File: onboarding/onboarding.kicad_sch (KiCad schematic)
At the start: 15 parts, among them IC1 ISL29125IROZ-T7, J1 Conn_01x05_Pin

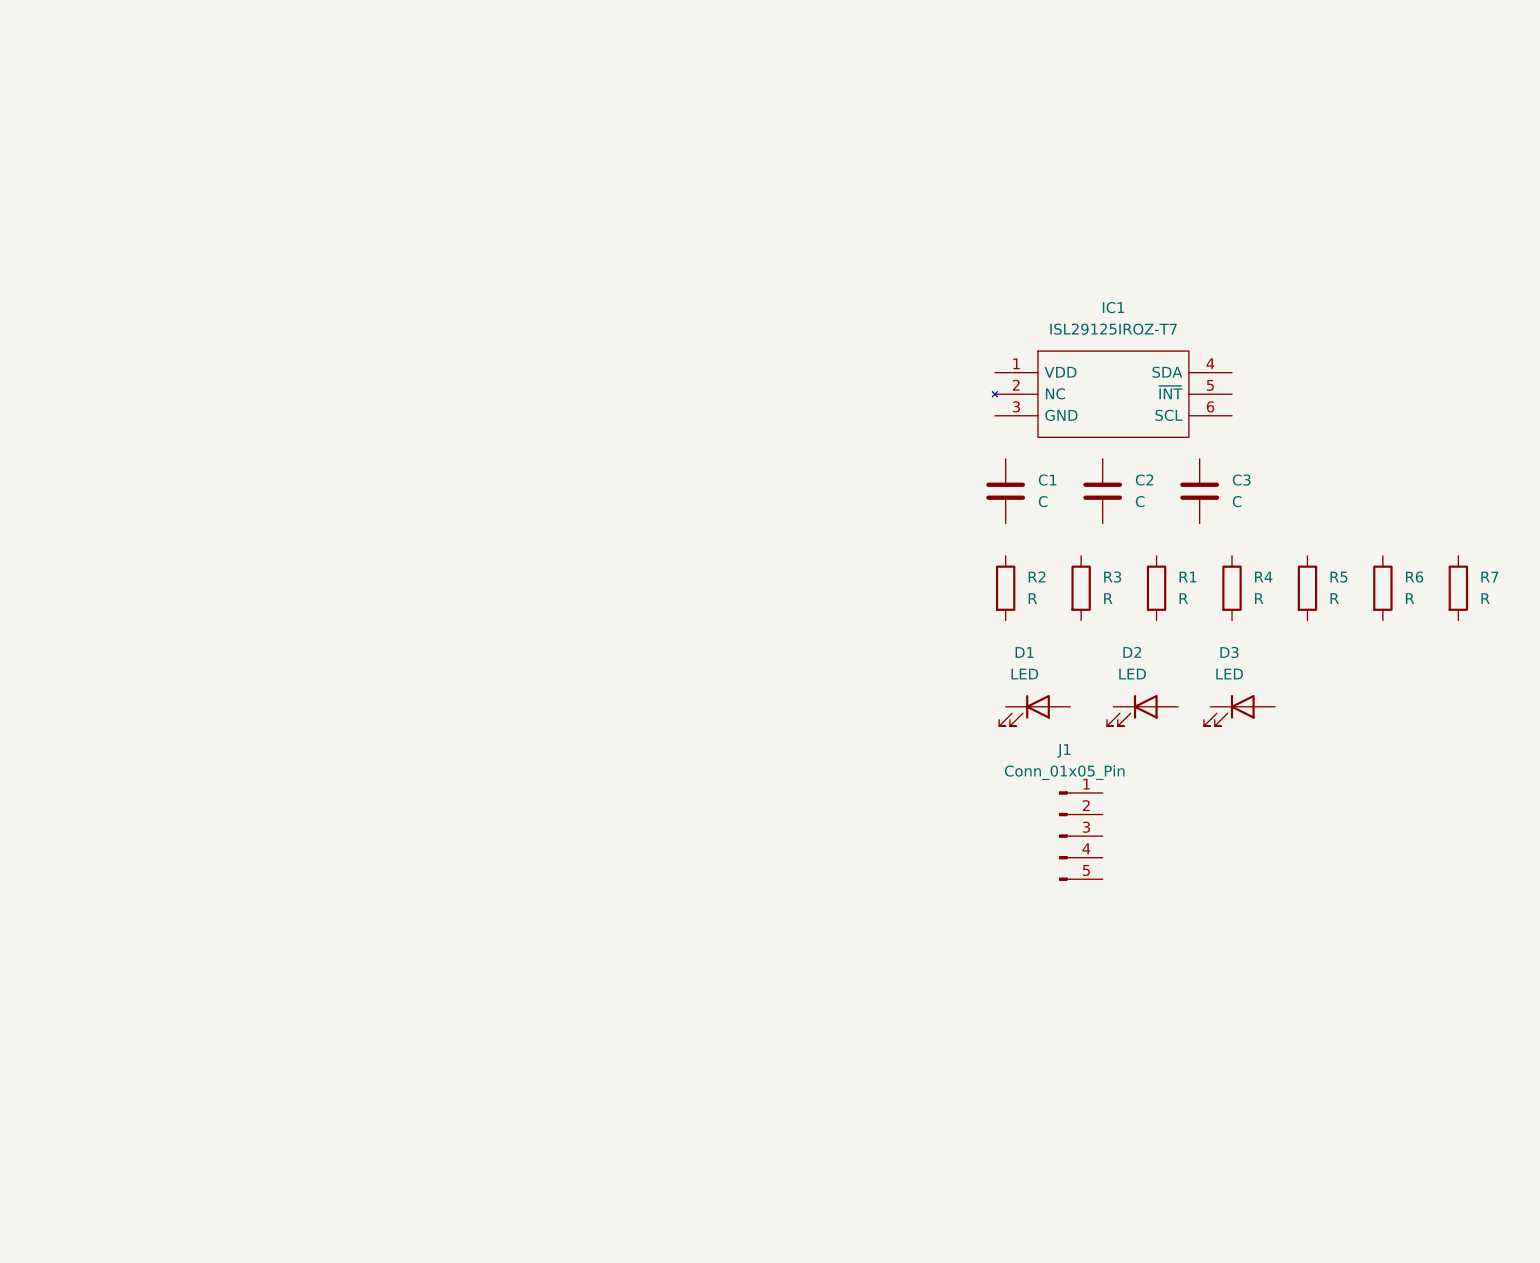
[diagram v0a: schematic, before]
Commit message: finished onboarding
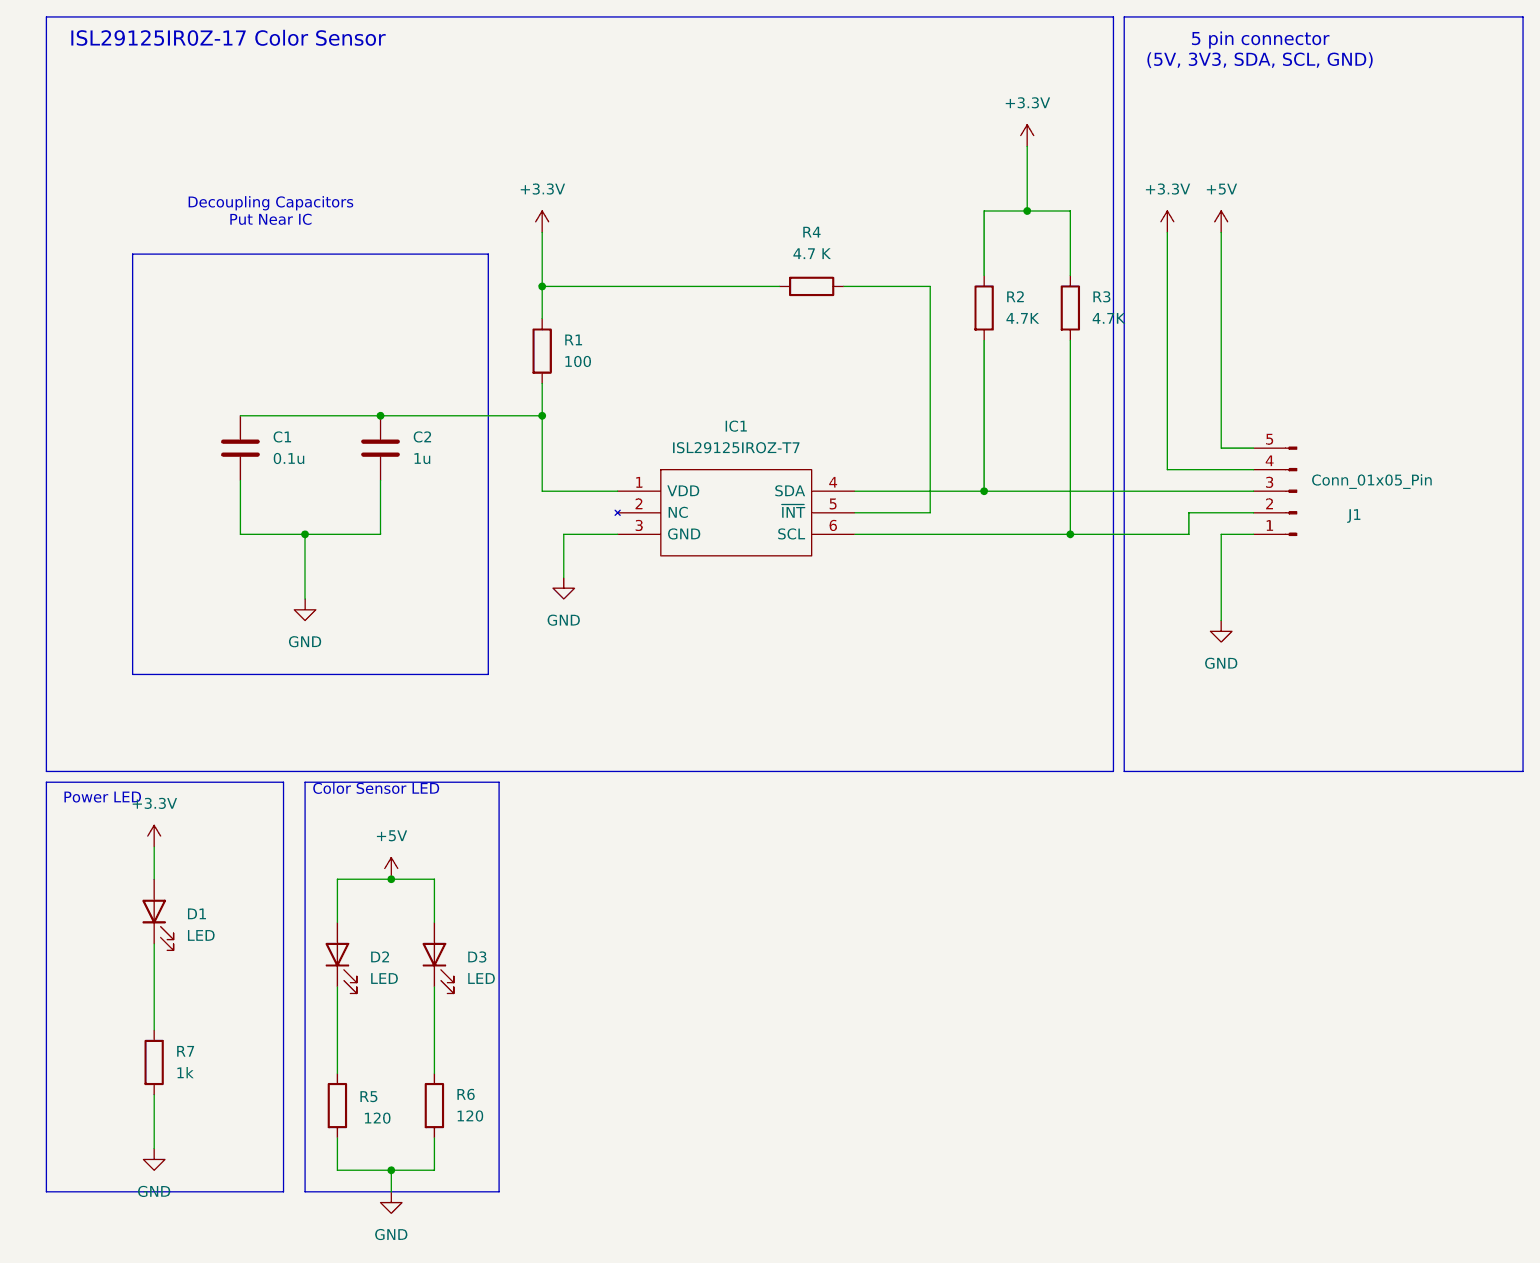
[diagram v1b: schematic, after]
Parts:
- removed C3: C, symbol Device:C
- C1: value C -> 0.1u; footprint (none) -> Capacitor_SMD:C_0603_1608Metric_Pad1.08x0.95mm_HandSolder
- C2: value C -> 1u; footprint (none) -> Capacitor_SMD:C_0603_1608Metric_Pad1.08x0.95mm_HandSolder
- D1: footprint (none) -> LED_SMD:LED_0603_1608Metric_Pad1.05x0.95mm_HandSolder
- D2, D3: footprint (none) -> LED_SMD:LED_0805_2012Metric_Pad1.15x1.40mm_HandSolder
- IC1: footprint ISL29125IROZT7 -> pcb_footprints:ISL29125IROZT7
- J1: footprint (none) -> Connector_PinHeader_2.54mm:PinHeader_1x05_P2.54mm_Horizontal
- R1: value R -> 100; footprint (none) -> Resistor_SMD:R_0603_1608Metric_Pad0.98x0.95mm_HandSolder
- R2, R3: value R -> 4.7K; footprint (none) -> Resistor_SMD:R_0603_1608Metric_Pad0.98x0.95mm_HandSolder
- R4: value R -> 4.7 K; footprint (none) -> Resistor_SMD:R_0603_1608Metric_Pad0.98x0.95mm_HandSolder
- R5, R6: value R -> 120; footprint (none) -> Resistor_SMD:R_0603_1608Metric_Pad0.98x0.95mm_HandSolder
- R7: value R -> 1k; footprint (none) -> Resistor_SMD:R_0603_1608Metric_Pad0.98x0.95mm_HandSolder
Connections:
- net at IC1.1 (VDD): now also C1.1, C2.1, R1.2
- net GND: now reaches IC1.3 (GND)
- net GND: now also C1.2, C2.2, J1.1 (Pin_1), R5.2, R6.2, R7.2
- net at IC1.4 (SDA): now also J1.3 (Pin_3), R2.2
- net at IC1.5 (~{INT}): now also R4.1
- net at IC1.6 (SCL): now also J1.2 (Pin_2), R3.2
- net at D1.1 (K): now also R7.1
- net +3.3V: now reaches D1.2 (A)
- net +3.3V: now also J1.4 (Pin_4), R1.1, R2.1, R3.1, R4.2
- net at D2.1 (K): now also R5.1
- net +5V: now reaches D2.2 (A)
- net +5V: now also D3.2 (A), J1.5 (Pin_5)
- net at R6.1: now also D3.1 (K)
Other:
- note added: "5 pin connector (5V, 3V3, SDA, SCL, GND)"
- note added: "Color Sensor LED"
- note added: "Decoupling Capacitors Put Near IC"
- note added: "ISL29125IR0Z-17 Color Sensor"
- note added: "Power LED"
- moved on the sheet: C1, C2, D1, D2, D3, IC1, J1, R1, R2, R3, R4, R5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
